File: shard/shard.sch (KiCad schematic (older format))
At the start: 3 parts, among them J0 Shard, J1 ISP

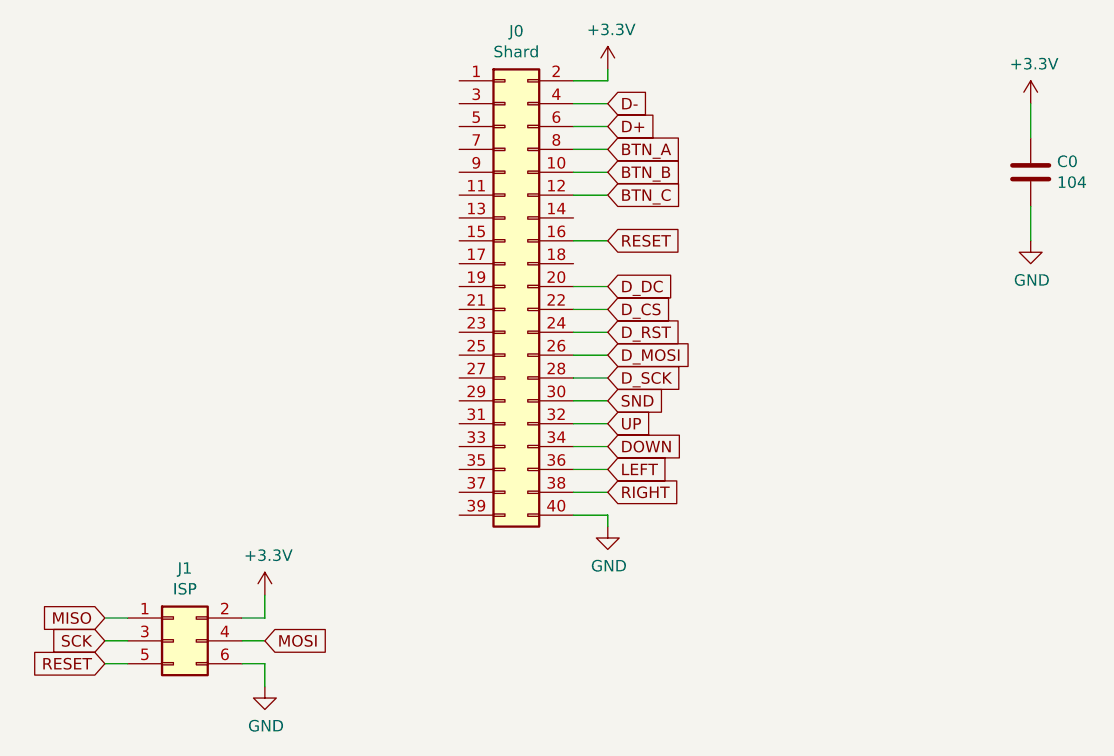
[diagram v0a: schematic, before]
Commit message: ::eyeroll::
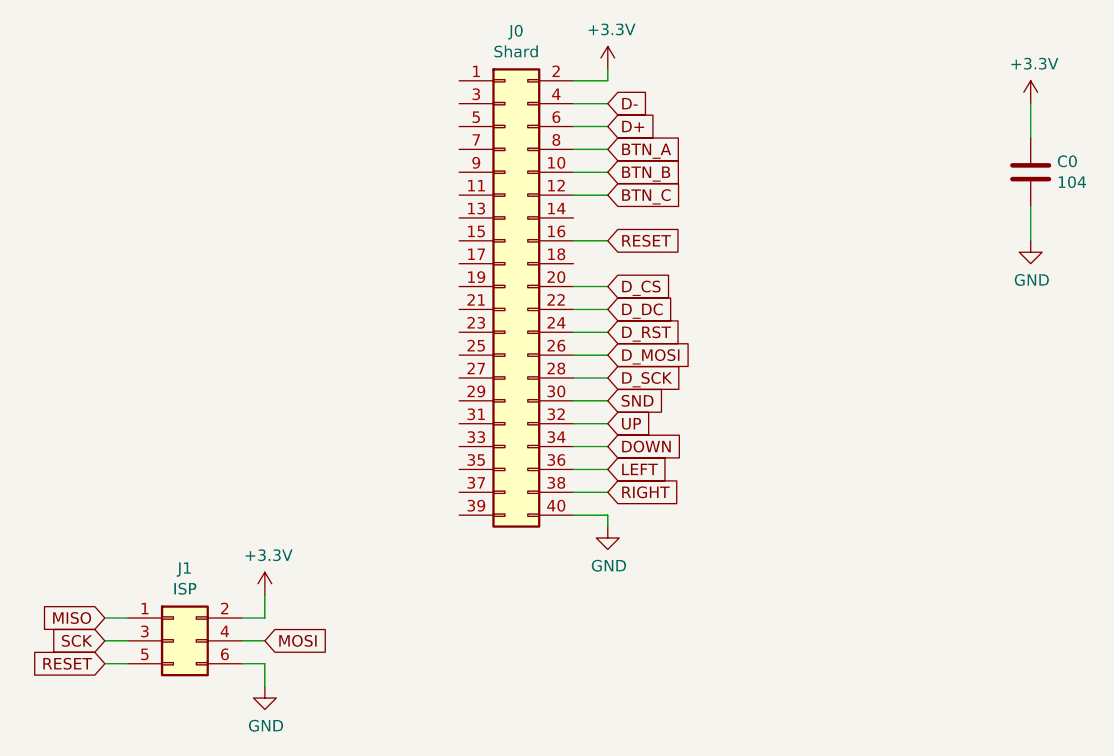
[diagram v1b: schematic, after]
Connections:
- net D_CS: now also J0.20 (Pin_20); no longer J0.22 (Pin_22)
- net D_DC: now also J0.22 (Pin_22); no longer J0.20 (Pin_20)
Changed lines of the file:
@@
 	1    0    0    -1
 $EndComp
+Text GLabel 5950 3550 2    50   Input ~ 0
+D_CS
 Text GLabel 5950 3650 2    50   Input ~ 0
-D_CS
-Text GLabel 5950 3550 2    50   Input ~ 0
 D_DC
 Text GLabel 5950 3750 2    50   Input ~ 0
